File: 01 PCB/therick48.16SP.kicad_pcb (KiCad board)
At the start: 2 copper layers, 308.9 x 75.8 mm, 181 parts, among them J1 TYPE-C-31-M12_13, J2 AVR-ISP-6_mod, K1 KEYSW, K10 KEYSW, K11 KEYSW, K12 KEYSW, K13 KEYSW, K14 KEYSW, K15 KEYSW, K16 KEYSW, K17 KEYSW, K18 KEYSW, K19 KEYSW, K2 KEYSW, K20 KEYSW, K21 KEYSW, K22 KEYSW, K23 KEYSW, K24 KEYSW, K25 KEYSW, K26 KEYSW, K27 KEYSW, K28 KEYSW, K29 KEYSW, K3 KEYSW, K30 KEYSW, K31 KEYSW, K32 KEYSW, K33 KEYSW, K34 KEYSW, K35 KEYSW, K36 KEYSW, K37 KEYSW, K38 KEYSW, K39 KEYSW, K4 KEYSW, K40 KEYSW, K41 KEYSW, K42 KEYSW, K43 KEYSW, K44 KEYSW, K45 KEYSW, K46 KEYSW, K47 KEYSW, K48 KEYSW, K49 KEYSW, K5 KEYSW, K50 KEYSW, K51 KEYSW, K52 KEYSW, K53 KEYSW, K54 KEYSW, K55 KEYSW, K56 KEYSW, K57 KEYSW, K58 KEYSW, K59 KEYSW, K6 KEYSW, K60 KEYSW, K61 KEYSW, K62 KEYSW, K63 KEYSW, K64 KEYSW, K7 KEYSW, K8 KEYSW, K9 KEYSW, SW1 SW_PUSH, SW2 Rotary_Encoder_Switch, U1 ATMEGA32U4, U10 HOLE, U11 HOLE, U2 HOLE, U3 USBLC6-2SC6, U4 HOLE, U5 HOLE, U6 HOLE, U7 HOLE, U8 HOLE, U9 HOLE, Y1 16MHz

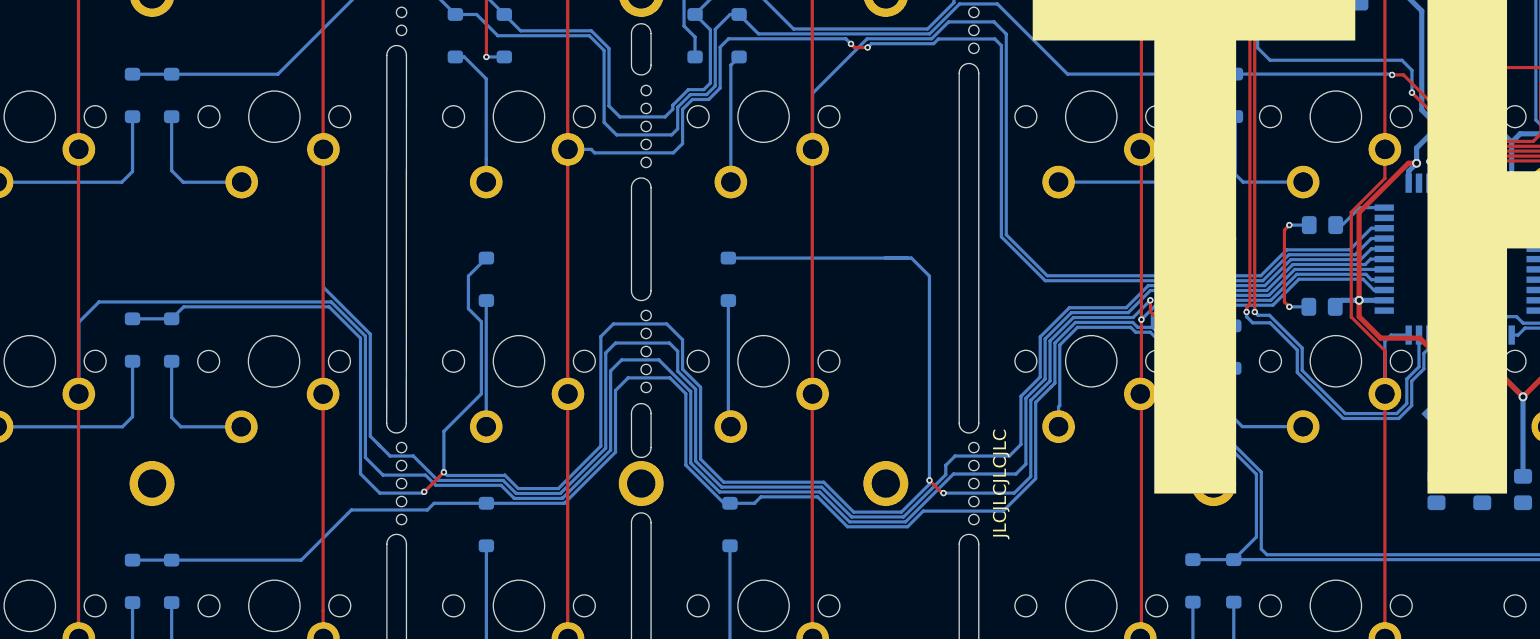
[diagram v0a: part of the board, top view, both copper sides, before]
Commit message: Update Gerbers
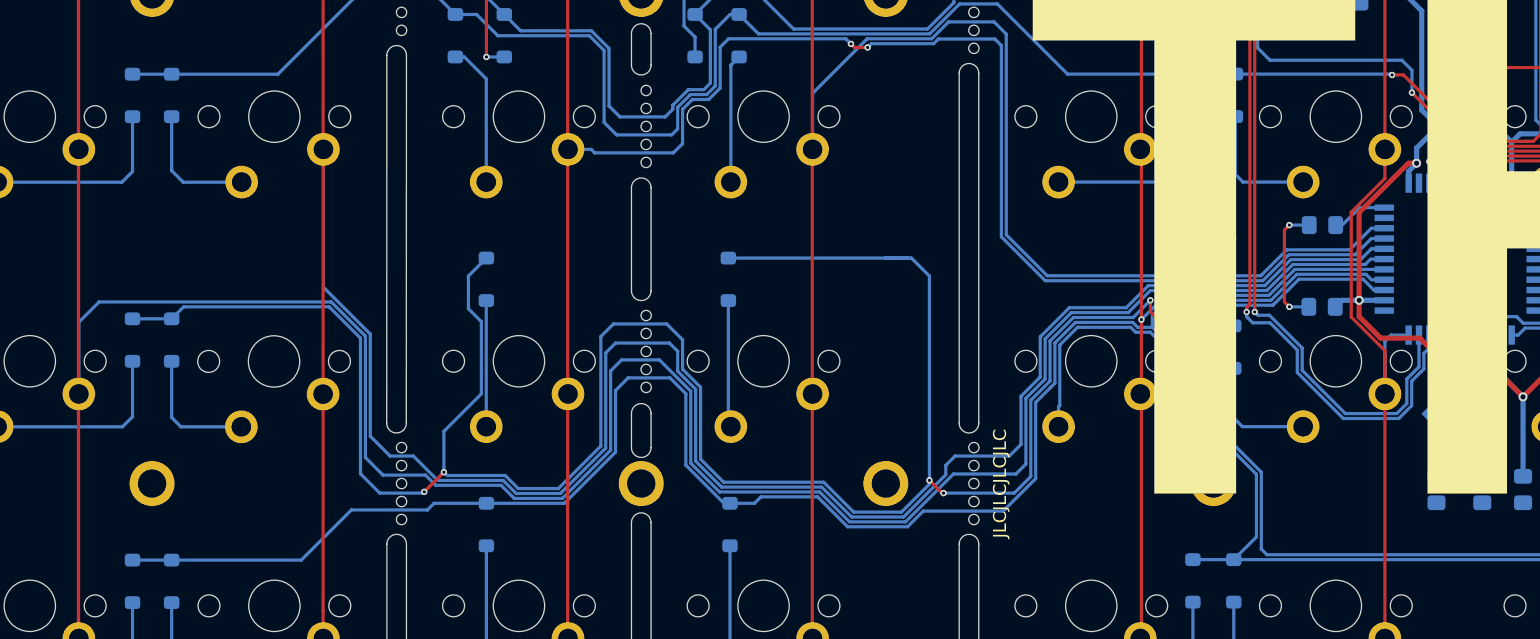
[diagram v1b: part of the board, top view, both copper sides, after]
